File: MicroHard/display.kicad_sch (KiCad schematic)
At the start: 14 parts, among them U5 MAX6955 Display Driver

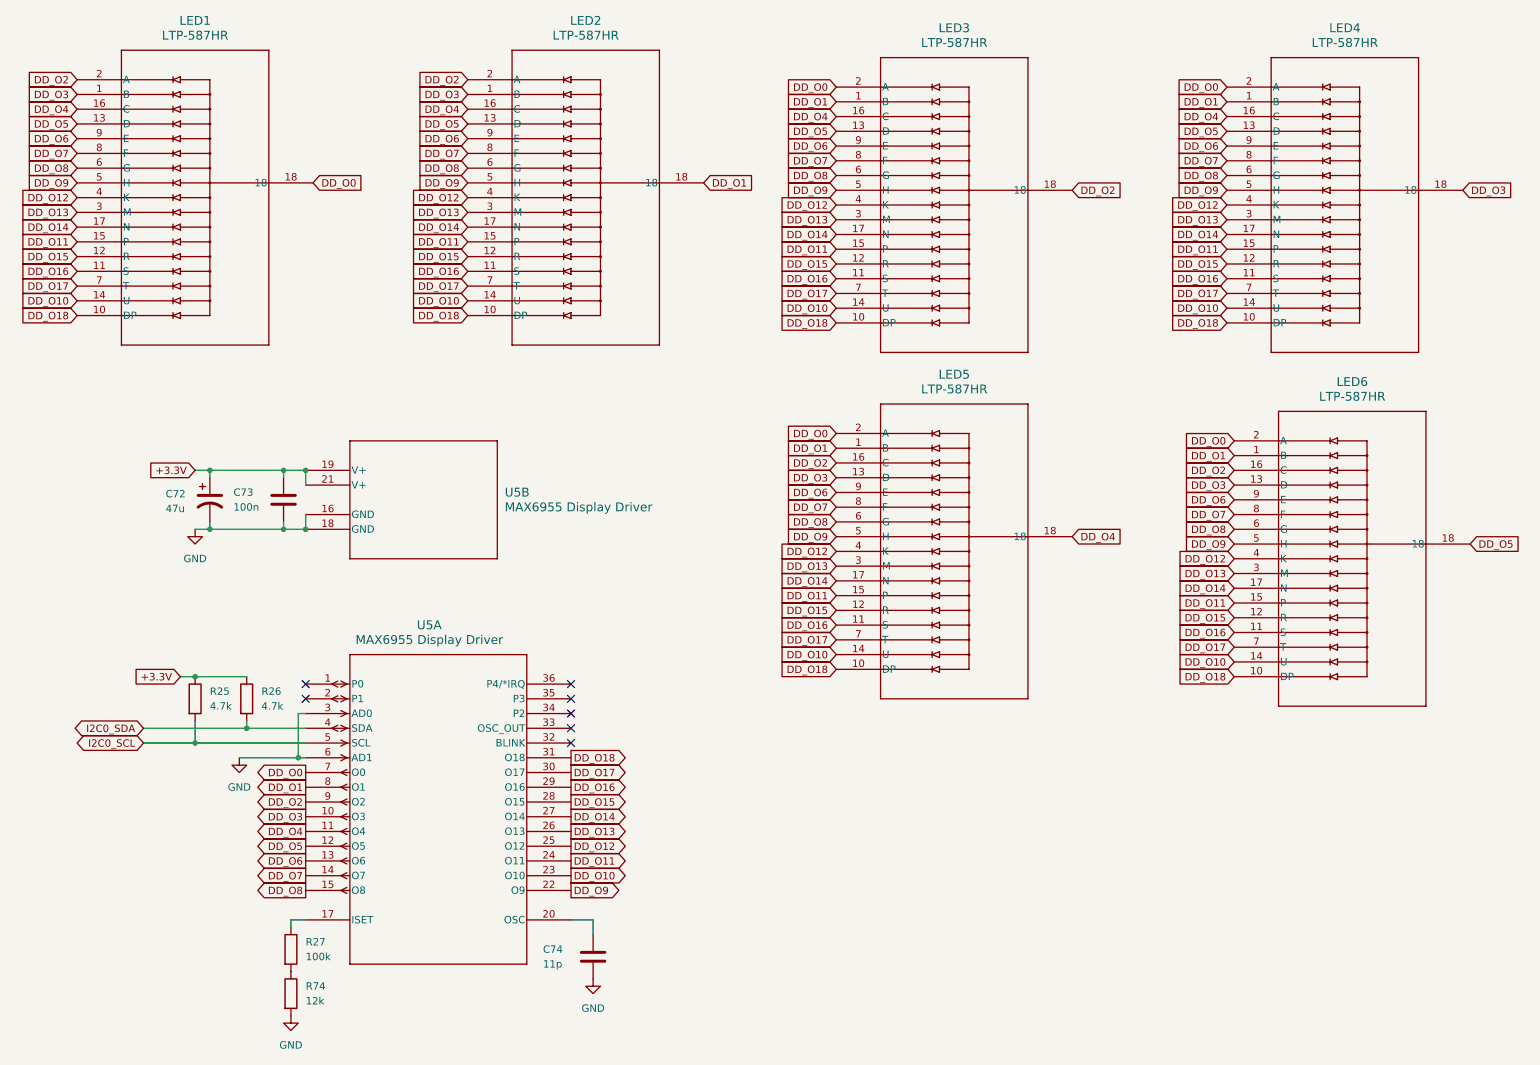
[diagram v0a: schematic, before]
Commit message: Fix schematics for delivery
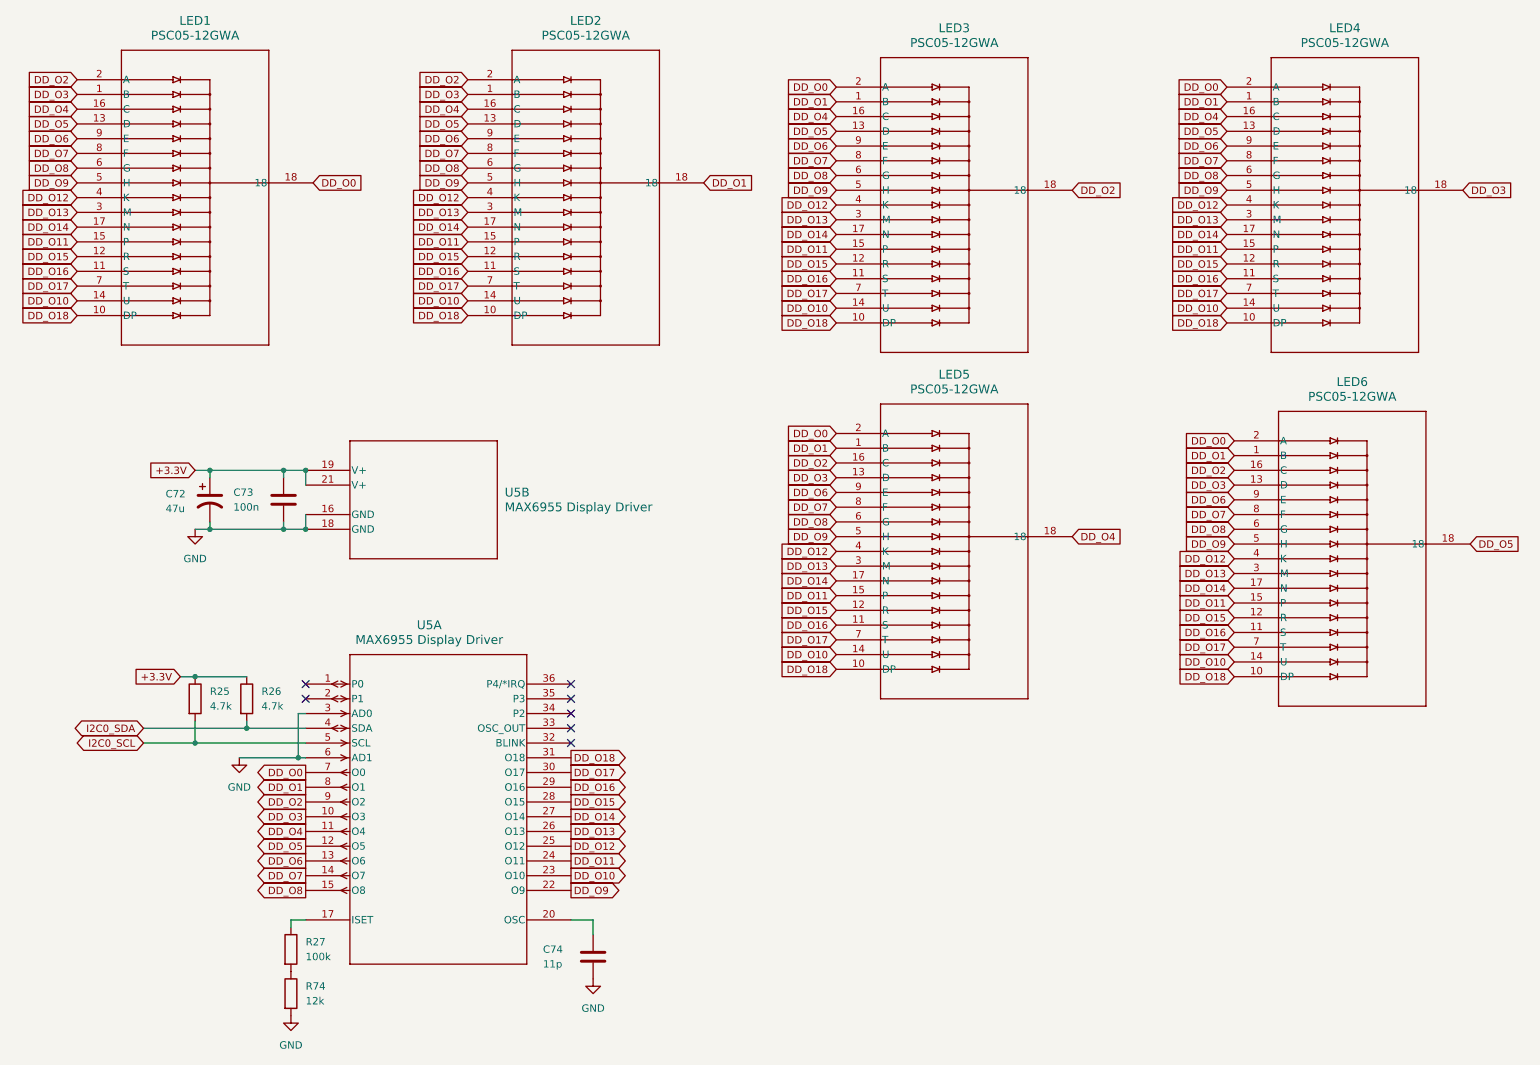
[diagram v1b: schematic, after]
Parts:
- removed LED1, LED2, LED3, LED4, LED5, LED6: LTP-587HR, LTP-587HR_LTO, symbol LTP-587HR:LTP-587HR
- added LED1, LED2, LED3, LED4, LED5, LED6: PSC05-12GWA, PSC05-12GWA_LTO, symbol PSC05-12GWA:PSC05-12GWA
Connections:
- net DD_O0: now also LED1.18, LED3.2 (A), LED4.2 (A), LED5.2 (A), LED6.2 (A)
- net DD_O1: now also LED2.18, LED3.1 (B), LED4.1 (B), LED5.1 (B), LED6.1 (B)
- net DD_O10: now also LED1.14 (U), LED2.14 (U), LED3.14 (U), LED4.14 (U), LED5.14 (U), LED6.14 (U)
- net DD_O11: now also LED1.15 (P), LED2.15 (P), LED3.15 (P), LED4.15 (P), LED5.15 (P), LED6.15 (P)
- net DD_O12: now also LED1.4 (K), LED2.4 (K), LED3.4 (K), LED4.4 (K), LED5.4 (K), LED6.4 (K)
- net DD_O13: now also LED1.3 (M), LED2.3 (M), LED3.3 (M), LED4.3 (M), LED5.3 (M), LED6.3 (M)
- net DD_O14: now also LED1.17 (N), LED2.17 (N), LED3.17 (N), LED4.17 (N), LED5.17 (N), LED6.17 (N)
- net DD_O15: now also LED1.12 (R), LED2.12 (R), LED3.12 (R), LED4.12 (R), LED5.12 (R), LED6.12 (R)
- net DD_O16: now also LED1.11 (S), LED2.11 (S), LED3.11 (S), LED4.11 (S), LED5.11 (S), LED6.11 (S)
- net DD_O17: now also LED1.7 (T), LED2.7 (T), LED3.7 (T), LED4.7 (T), LED5.7 (T), LED6.7 (T)
- net DD_O18: now also LED1.10 (DP), LED2.10 (DP), LED3.10 (DP), LED4.10 (DP), LED5.10 (DP), LED6.10 (DP)
- net DD_O2: now also LED1.2 (A), LED2.2 (A), LED3.18, LED5.16 (C), LED6.16 (C)
- net DD_O3: now also LED1.1 (B), LED2.1 (B), LED4.18, LED5.13 (D), LED6.13 (D)
- net DD_O4: now also LED1.16 (C), LED2.16 (C), LED3.16 (C), LED4.16 (C), LED5.18
- net DD_O5: now also LED1.13 (D), LED2.13 (D), LED3.13 (D), LED4.13 (D), LED6.18
- net DD_O6: now also LED1.9 (E), LED2.9 (E), LED3.9 (E), LED4.9 (E), LED5.9 (E), LED6.9 (E)
- net DD_O7: now also LED1.8 (F), LED2.8 (F), LED3.8 (F), LED4.8 (F), LED5.8 (F), LED6.8 (F)
- net DD_O8: now also LED1.6 (G), LED2.6 (G), LED3.6 (G), LED4.6 (G), LED5.6 (G), LED6.6 (G)
- net DD_O9: now also LED1.5 (H), LED2.5 (H), LED3.5 (H), LED4.5 (H), LED5.5 (H), LED6.5 (H)
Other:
- company: (none) -> MicroHard
- title: (none) -> Alphanumeric Display
